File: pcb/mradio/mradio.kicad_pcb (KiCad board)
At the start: 6 copper layers, 132.2 x 75 mm, 191 parts, among them J101 Conn_02x07_Odd_Even, J202 Conn_01x02, J301 2250065-1, J401 MM60-52B1-E1-R650, J501 MDT420E01001, Q101 Q_NMOS, Q102 Q_NMOS, Q103 Q_NMOS, Q104 Q_NMOS, Q105 Q_NMOS, Q106 Q_NMOS, Q107 Q_NMOS, Q108 Q_NMOS, Q301 SSM3K56FS_LF, U1 STM32H745ZITx, U301 DP83825I, U401 74AVC4T774, U402 74AVC4T774, U502 SN74LVC1T45DRL, U601 TPS54560BDDA, U701 TPS54560BDDA, U801 TPS7A8500ARGRR, U901 TPS7A8500ARGRR, Y301 DSC1525JL2A-25M00000T

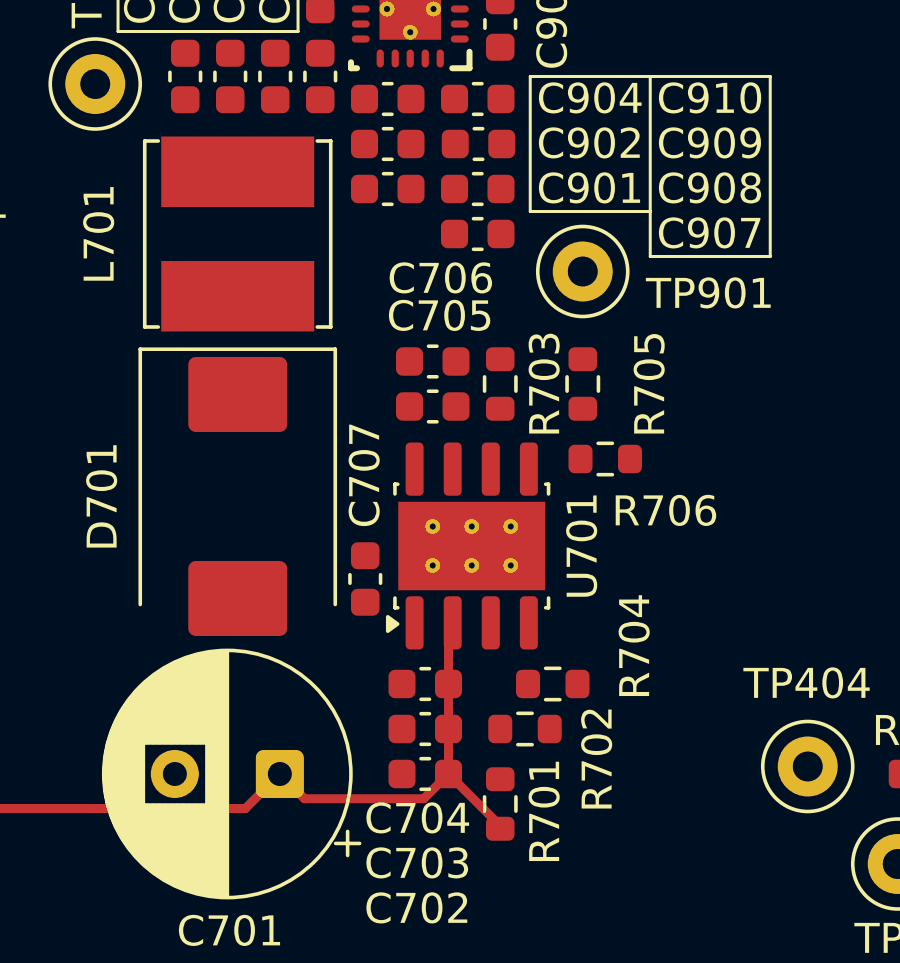
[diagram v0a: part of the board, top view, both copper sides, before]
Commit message: Changed 2v2 testpoint net to actually be 2v2...
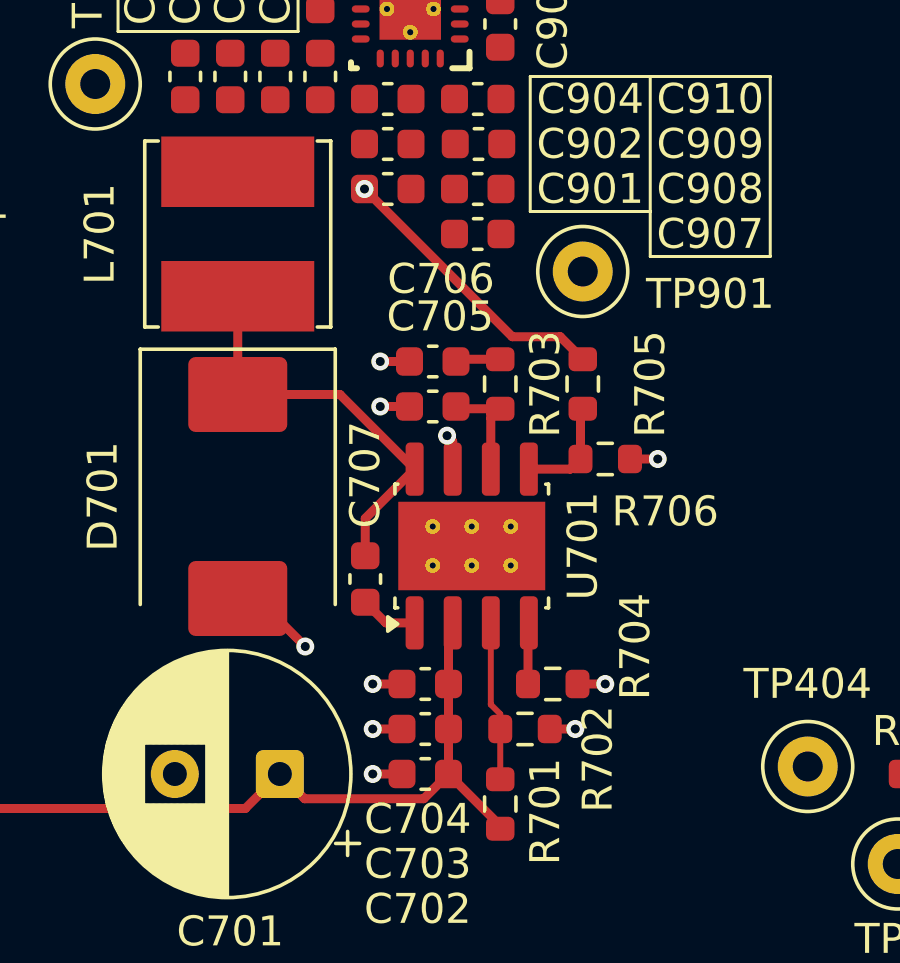
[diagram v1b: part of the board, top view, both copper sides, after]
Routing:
- net Net-(D701-K): track 0.00 -> 13.8 mm
- net GND: track 150.5 -> 162.2 mm, vias 128 -> 138
- net +2V2: track 0.00 -> 9.63 mm, vias 0 -> 1
- net Net-(U701-EN): track 0.00 -> 5.34 mm
- net Net-(U701-COMP): track 0.00 -> 3.65 mm
- net /Power Distribution/2v2_Buck/FB: track 0.00 -> 3.57 mm
- net Net-(U701-RT/CLK): track 0.00 -> 2.05 mm
- net Net-(U701-BOOT): track 0.00 -> 1.93 mm
- net Net-(C706-Pad1): track 0.00 -> 1.51 mm
